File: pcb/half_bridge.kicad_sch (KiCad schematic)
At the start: 23 parts, among them U5 IKW40N120H3, U6 IKW40N120H3, U7 UCC21550BDW, U8 SS14

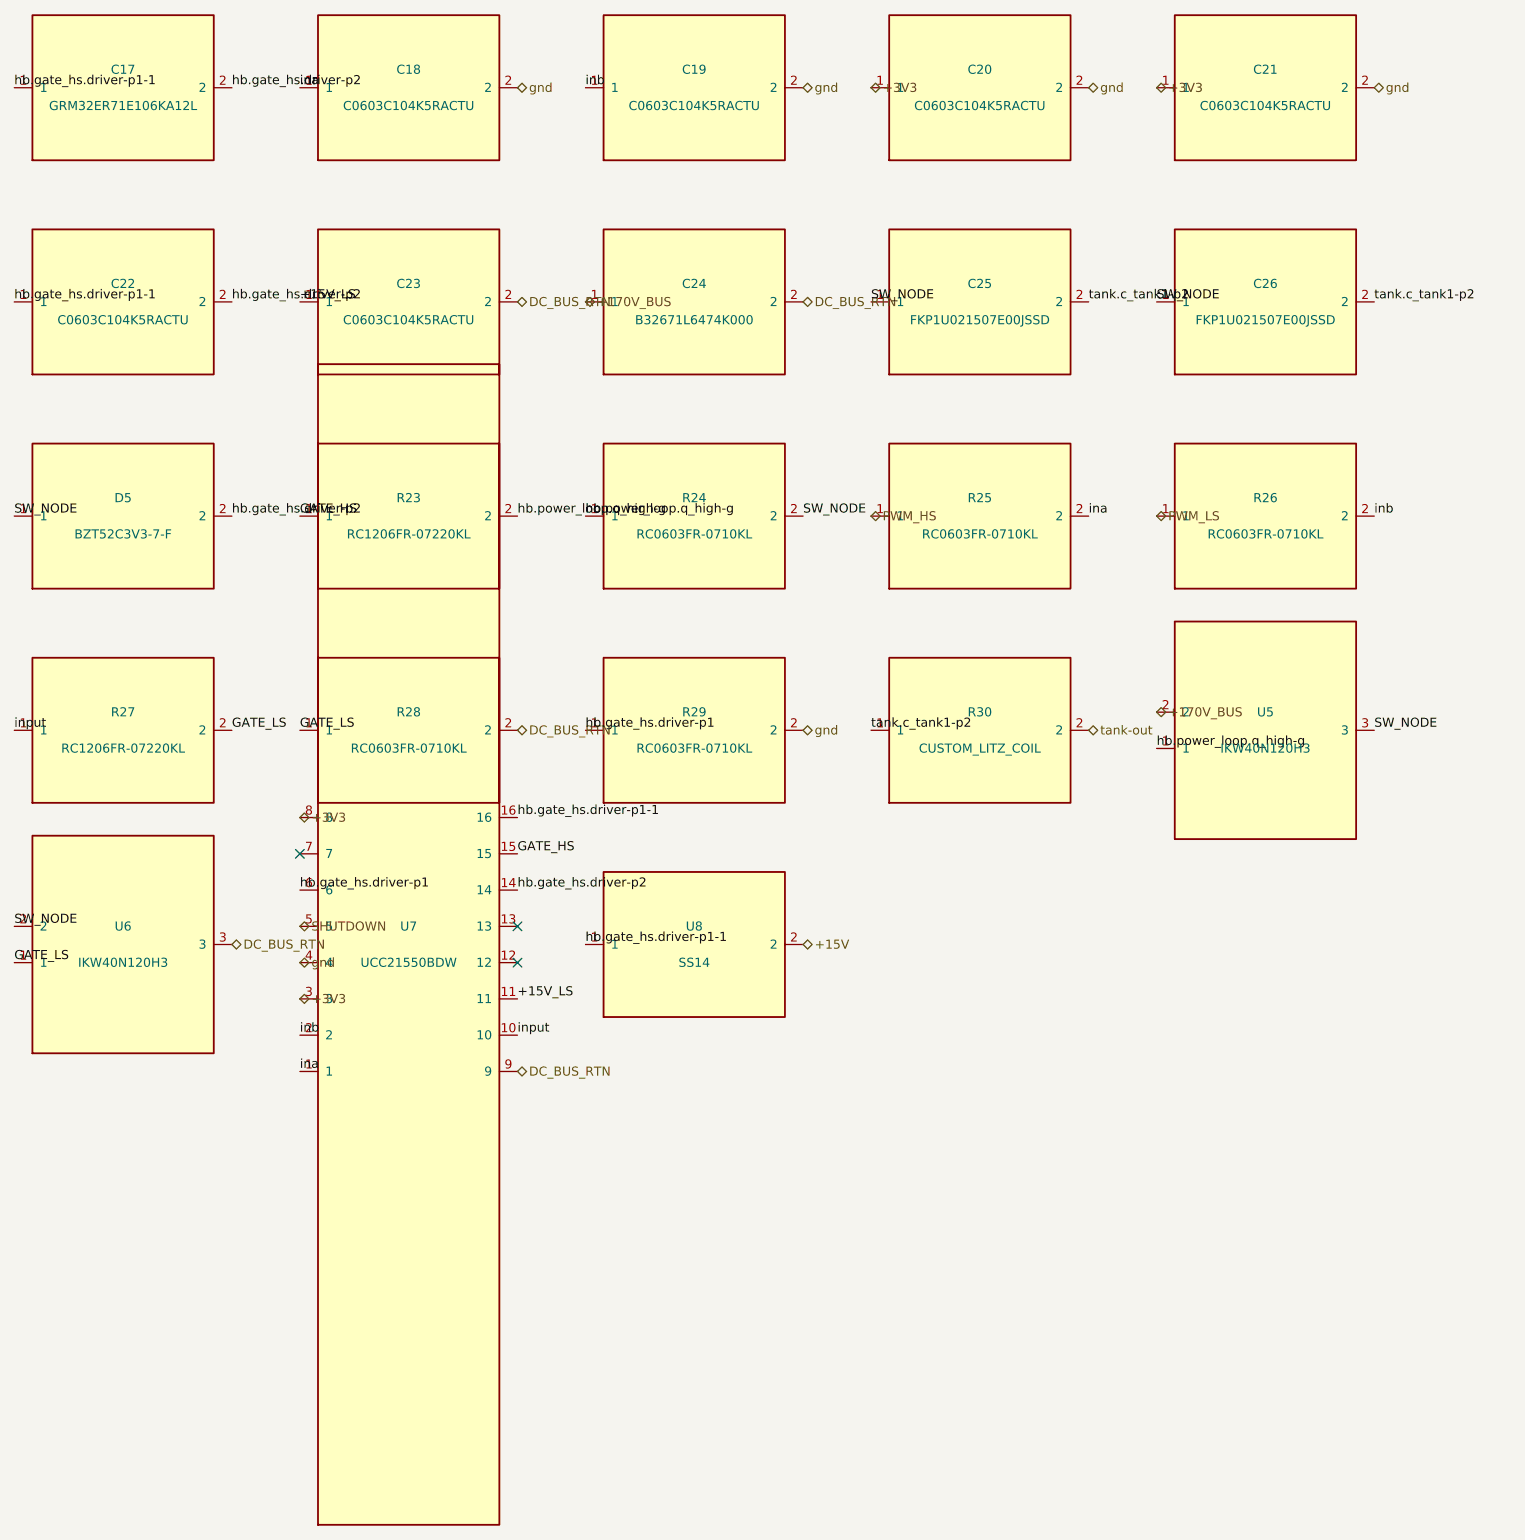
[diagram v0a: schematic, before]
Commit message: fix: refresh generated schematics after source reconciliation
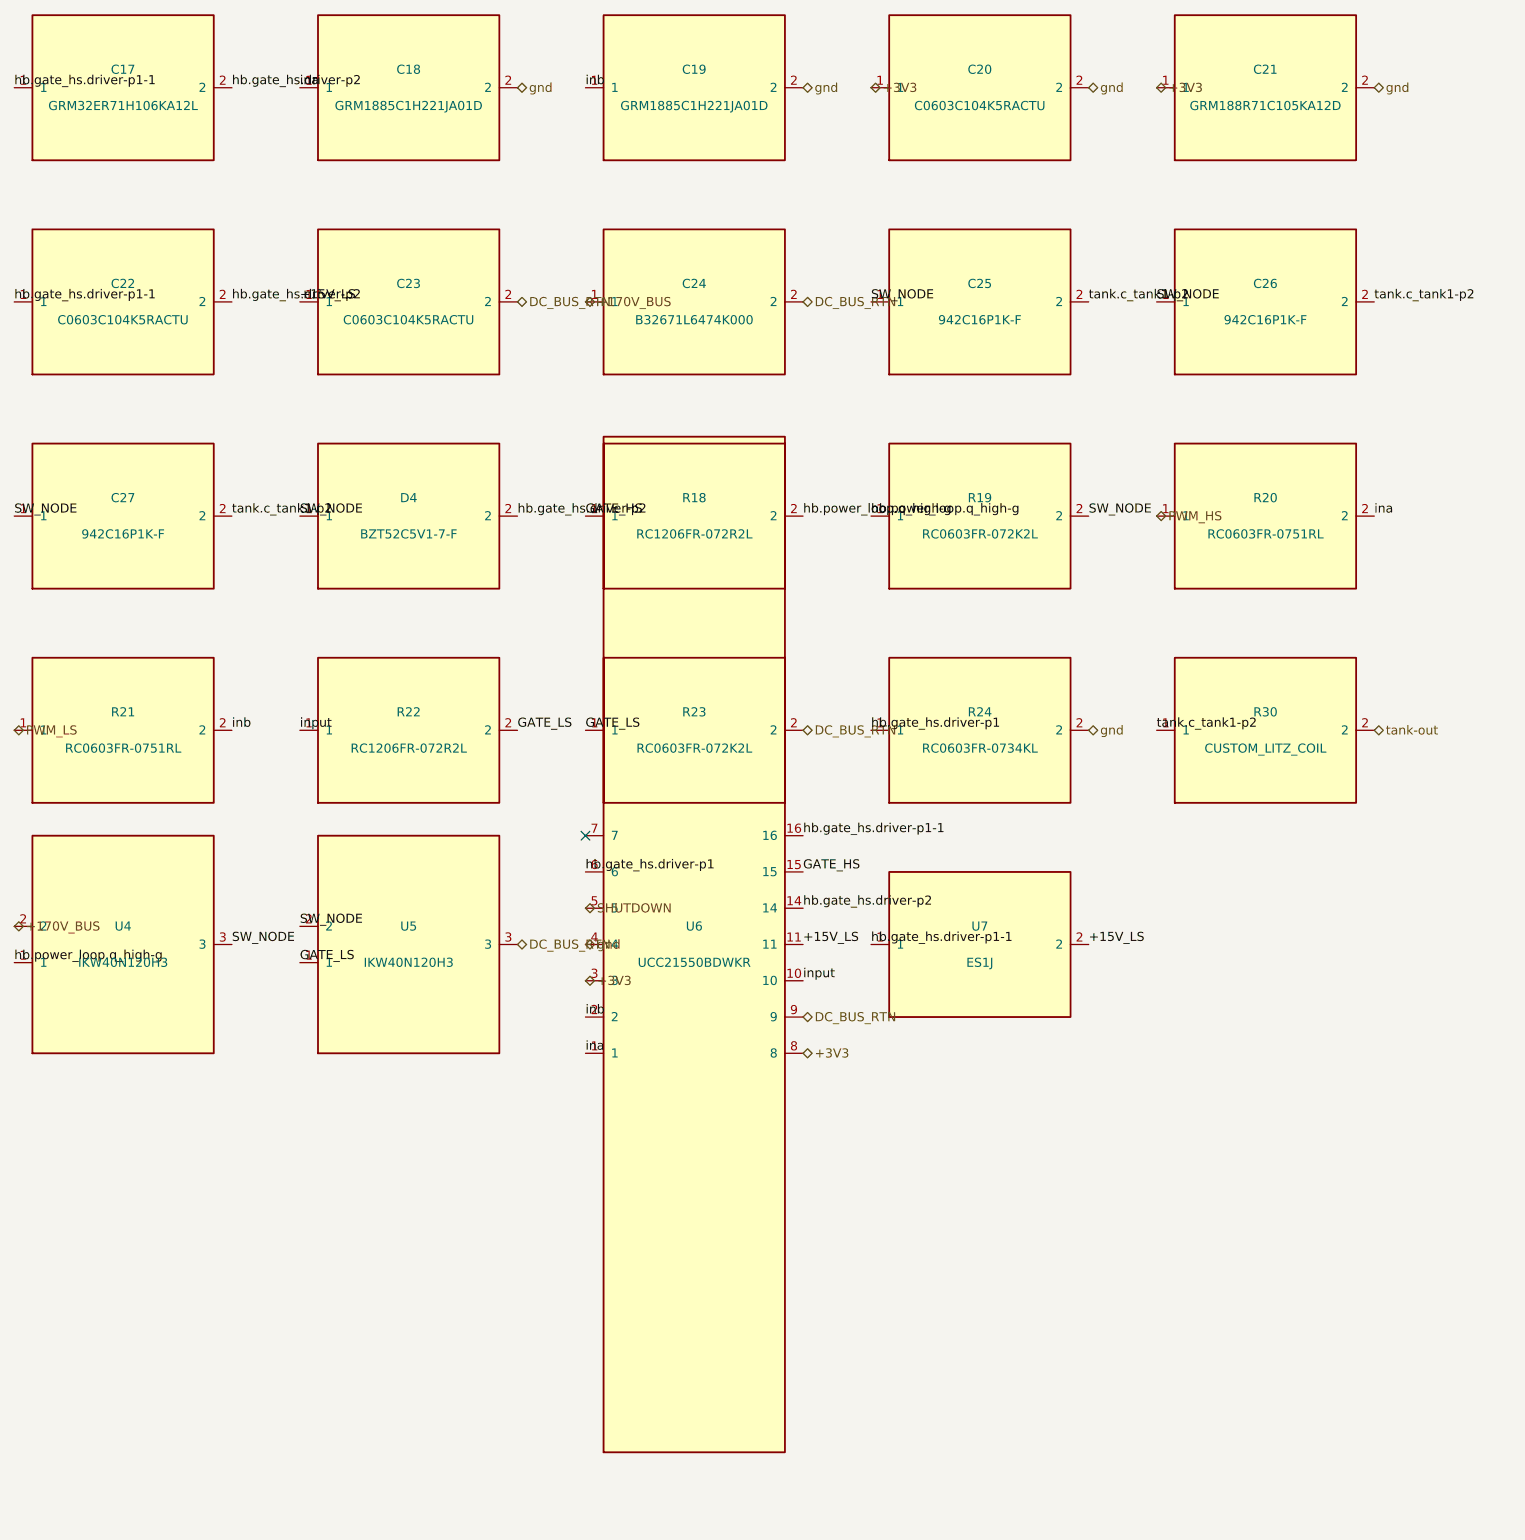
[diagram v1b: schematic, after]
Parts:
- added C27: 942C16P1K-F, temper:C_Axial_L34.0mm_D22.5mm_P40.00mm_Horizontal, symbol 942C16P1K-F
- C17: value GRM32ER71E106KA12L -> GRM32ER71H106KA12L
- C18, C19: value C0603C104K5RACTU -> GRM1885C1H221JA01D
- C21: value C0603C104K5RACTU -> GRM188R71C105KA12D
- C25, C26: value FKP1U021507E00JSSD -> 942C16P1K-F; footprint Capacitor_THT:C_Rect_L31.5mm_W13.0mm_P27.50mm_MKS4 -> temper:C_Axial_L34.0mm_D22.5mm_P40.00mm_Horizontal; symbol FKP1U021507E00JSSD -> 942C16P1K-F
- D4: renamed from D5; value BZT52C3V3-7-F -> BZT52C5V1-7-F; symbol BZT52C3V3-7-F -> BZT52C5V1-7-F
- R18: renamed from R23; value RC1206FR-07220KL -> RC1206FR-072R2L; symbol RC1206FR-07220KL -> RC1206FR-07100RL
- R19: renamed from R24; value RC0603FR-0710KL -> RC0603FR-072K2L; symbol RC0603FR-0710KL -> RC0603FR-07100KL
- R20: renamed from R25; value RC0603FR-0710KL -> RC0603FR-0751RL; symbol RC0603FR-0710KL -> RC0603FR-07100KL
- R21: renamed from R26; value RC0603FR-0710KL -> RC0603FR-0751RL; symbol RC0603FR-0710KL -> RC0603FR-07100KL
- R22: renamed from R27; value RC1206FR-07220KL -> RC1206FR-072R2L; symbol RC1206FR-07220KL -> RC1206FR-07100RL
- R23: renamed from R28; value RC0603FR-0710KL -> RC0603FR-072K2L; symbol RC0603FR-0710KL -> RC0603FR-07100KL
- R24: renamed from R29; value RC0603FR-0710KL -> RC0603FR-0734KL; symbol RC0603FR-0710KL -> RC0603FR-07100KL
- U6: renamed from U7; value UCC21550BDW -> UCC21550BDWKR; symbol UCC21550BDW -> UCC21550BDWKR
- U7: renamed from U8; value SS14 -> ES1J
- renumbered U5 to U4, U6 to U5
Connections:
- net +15V is gone; now on net +15V_LS: U7.2
- net SW_NODE: now also C27.1
- net tank.c_tank1-p2: now also C27.2
- no-connect marks 3 -> 1
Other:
- moved on the sheet: D4, R18, R19, R20, R21, R22, R23, R24, R30, U4, U5, U7
